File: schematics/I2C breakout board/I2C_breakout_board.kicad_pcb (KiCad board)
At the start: 2 copper layers, 16.3 x 19.6 mm, 7 parts, among them J1 Conn_01x07_Pin, J2 Conn_01x07_Pin, U1 ENS210-LQFM, U2 OPT4001DTSR

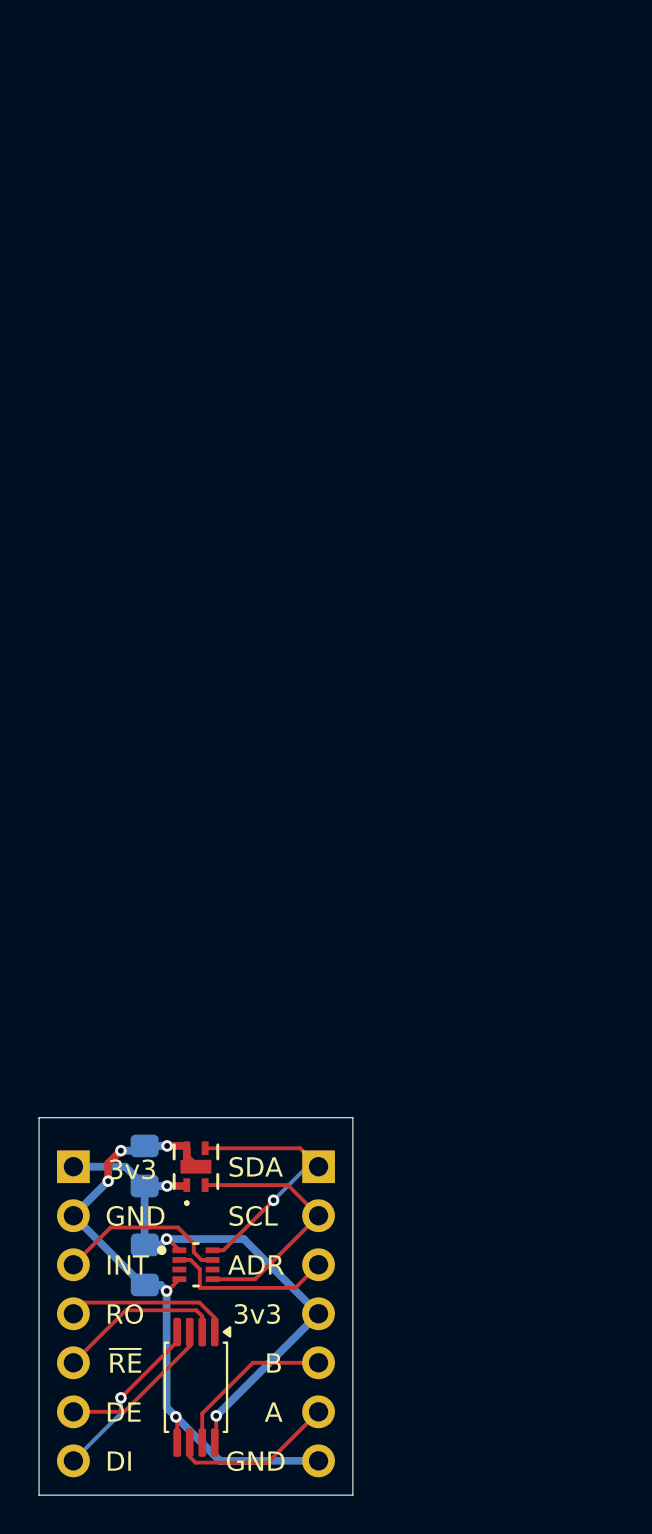
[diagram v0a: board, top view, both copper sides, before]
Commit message: final version of air sensors breakout board
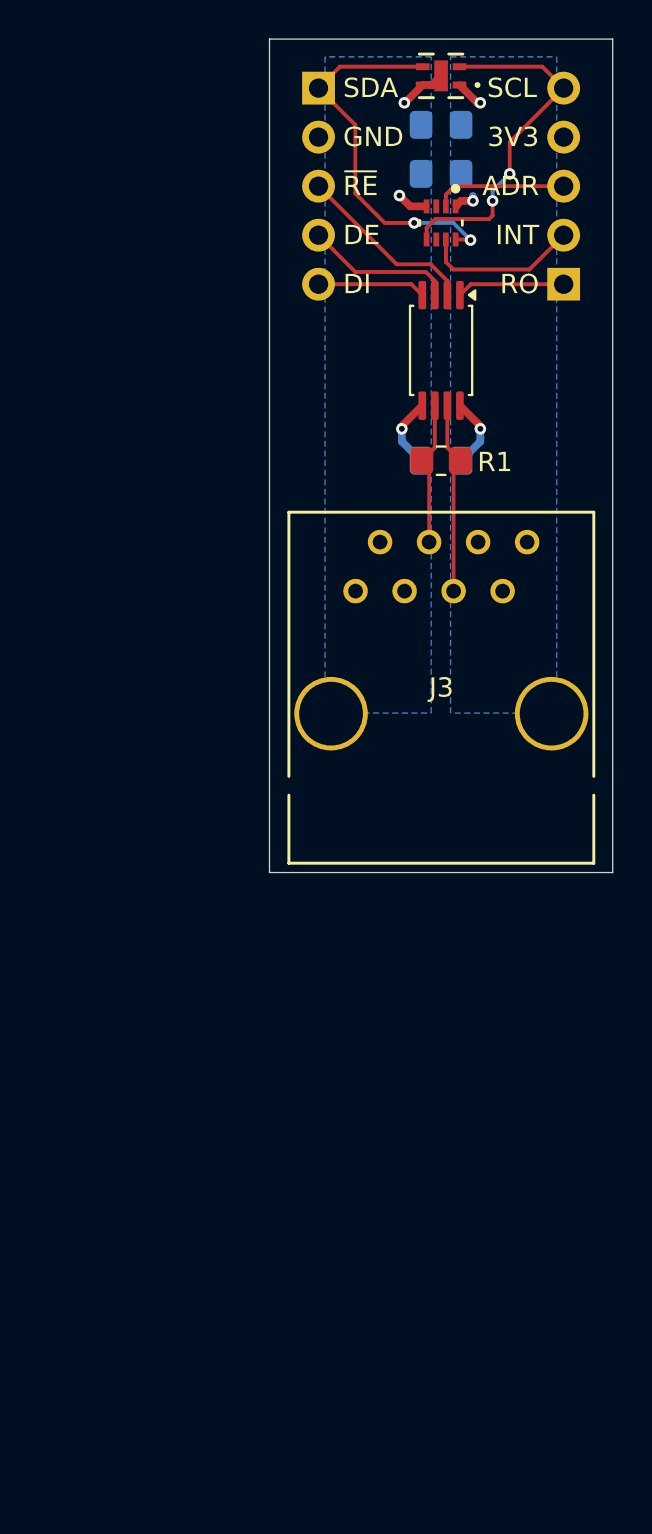
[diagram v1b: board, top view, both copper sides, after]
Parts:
- removed J1, J2: Conn_01x07_Pin, Connector_PinHeader_2.54mm:PinHeader_1x07_P2.54mm_Vertical
- added C3: 0.1u, Capacitor_SMD:C_0805_2012Metric_Pad1.18x1.45mm_HandSolder, B.Cu at (143.5, 90.4)
- added J3: 54602-908LF, 54602_908LF_footprints:CONN8_2-908LF_AMP, F.Cu at (139.1, 97.2)
- added J4: Conn_01x05_Pin, Connector_PinHeader_2.54mm:PinHeader_1x05_P2.54mm_Vertical, B.Cu at (137.2, 71.1)
- added J5: Conn_01x05_Pin, Connector_PinHeader_2.54mm:PinHeader_1x05_P2.54mm_Vertical, B.Cu at (149.9, 81.3)
- added R1: 120, Resistor_SMD:R_0805_2012Metric_Pad1.20x1.40mm_HandSolder, F.Cu at (143.5, 90.4)
- moved C2 61.0 mm to (143.5, 73.0), turned to 0 degrees
- moved U1 57.9 mm to (143.5, 70.5), turned to 180 degrees
- moved U2 55.4 mm to (143.5, 78.1), turned to -90 degrees
- moved U3 55.2 mm to (143.5, 84.7)
- moved C1 53.6 mm to (143.5, 75.6), turned to 180 degrees
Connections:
- net U3_GND renamed GND
- U3 pad 6: U3_A -> Net-(U3-A)
- U3 pad 7: U3__B -> Net-(U3-B)
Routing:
- net GND: track 32.9 -> 8.05 mm, vias 5 -> 3
- net +3.3V: track 29.9 -> 7.09 mm
- net Net-(U3-B): track 0.00 -> 10.0 mm
- net U3_A: track 8.63 -> 0.00 mm
- net U3__B: track 8.62 -> 0.00 mm
- net Net-(U3-A): track 0.00 -> 7.50 mm
- net SDA: track 13.6 -> 19.9 mm, vias 1 -> 2
- net SCL: track 13.4 -> 18.3 mm, vias 0 -> 2
- net U3_DI: track 8.90 -> 5.61 mm, vias 1 -> 0
- net U3_RO: track 8.75 -> 5.61 mm
- net U2_ADDR: track 8.88 -> 6.89 mm
- net U2_INT: track 9.11 -> 8.16 mm
- net U3_DE: track 8.61 -> 7.74 mm
- net U3_/RE: track 8.75 -> 9.45 mm
- added copper zone on B.Cu, net +3.3V
- added copper zone on B.Cu, net GND
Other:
- board size 16.3 x 19.6 mm -> 17.8 x 43.2 mm
- board text added: "3V3"
- board text removed: "3v3"
- board text removed: "A"
- board text removed: "B"
